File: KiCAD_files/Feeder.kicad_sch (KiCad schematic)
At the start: 61 parts, among them J505 Conn_01x03, Q501 60V N channel, Q502 TK13P25D,RQ, Q503 Q_Dual_NMOS_G1S2G2D2S1D1, Q504 Q_Dual_NMOS_G1S2G2D2S1D1, T501 PA2467NL, U501 NCP12700, U502 HMHA2801A, U503 TL431MFDT,215

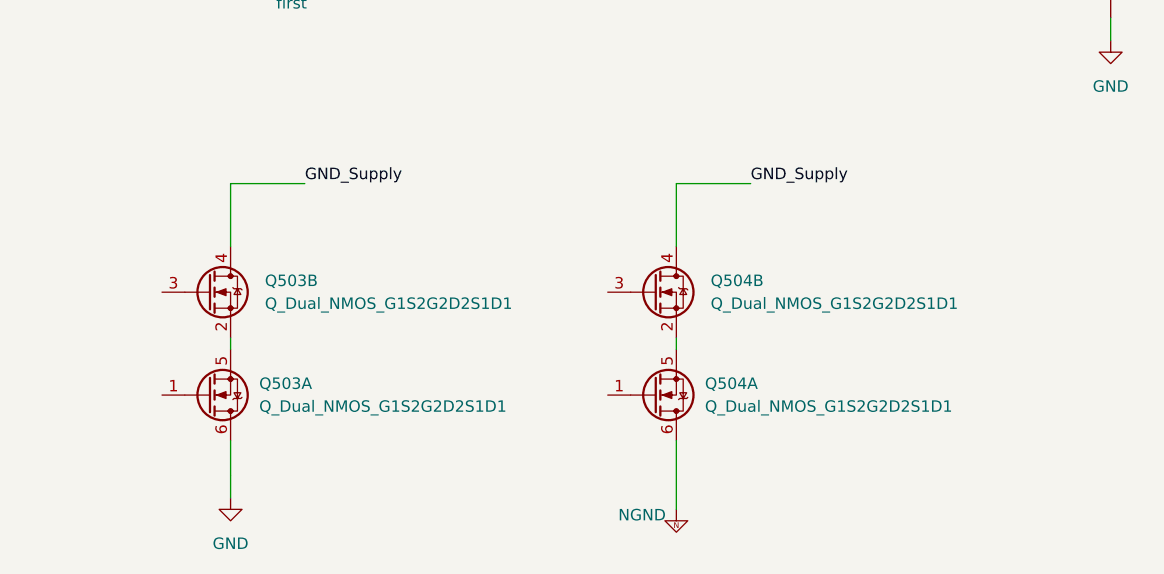
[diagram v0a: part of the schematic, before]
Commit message: Feature Freeze PCB ordered
Former-commit-id: 656e77d39b103ec58b17965582500bfb0a5b80a0
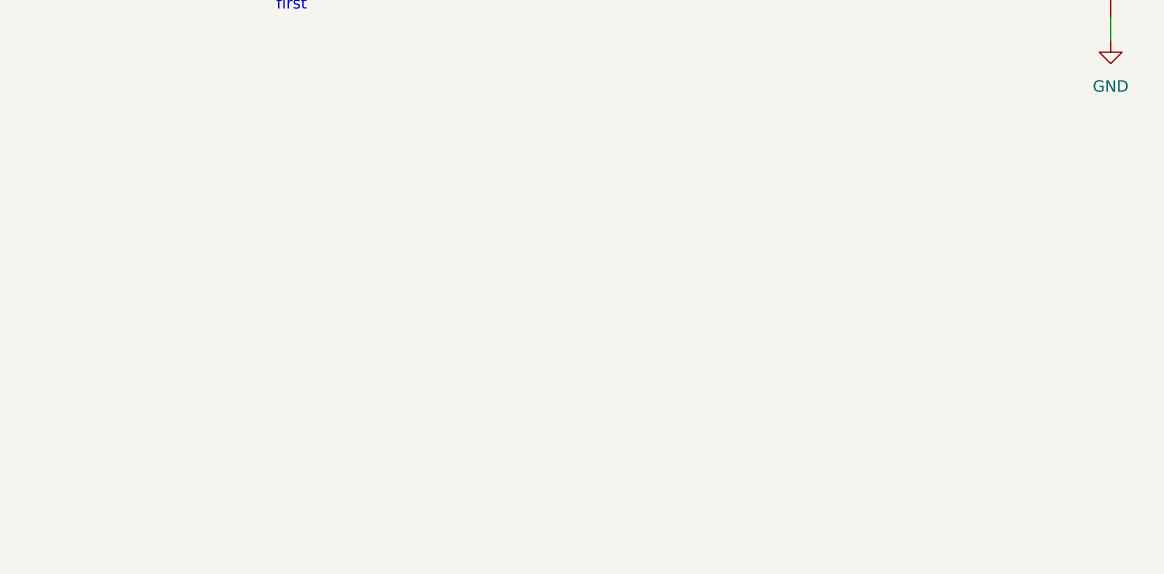
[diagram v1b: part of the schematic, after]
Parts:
- removed Q503, Q504: Q_Dual_NMOS_G1S2G2D2S1D1, symbol Device:Q_Dual_NMOS_G1S2G2D2S1D1
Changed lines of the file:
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@@
-    (stroke (width 0) (type default) (color 0 0 0 0))
-  )
-  (wire (pts (xy 71.755 223.52) (xy 71.755 224.79))
     (stroke (width 0) (type default) (color 0 0 0 0))
   )
@@
     (stroke (width 0) (type default) (color 0 0 0 0))
   )
-  (wire (pts (xy 121.285 234.95) (xy 121.285 238.76))
-    (stroke (width 0) (type default) (color 0 0 0 0))
-  )
   (wire (pts (xy 113.03 88.265) (xy 113.03 75.565))
     (stroke (width 0) (type default) (color 0 0 0 0))
@@
   )
   (wire (pts (xy 237.49 103.505) (xy 237.49 104.775))
-    (stroke (width 0.45) (type default) (color 0 0 0 0))
-  )
-  (wire (pts (xy 121.285 238.76) (xy 121.285 241.3))
     (stroke (width 0.45) (type default) (color 0 0 0 0))
   )
@@
     (stroke (width 0) (type default) (color 0 0 0 0))
   )
-  (wire (pts (xy 71.755 206.375) (xy 80.01 206.375))
-    (stroke (width 0) (type default) (color 0 0 0 0))
-  )
   (wire (pts (xy 196.85 104.775) (xy 205.105 104.775))
     (stroke (width 0) (type default) (color 0 0 0 0))
@@
     (stroke (width 0) (type default) (color 0 0 0 0))
   )
-  (wire (pts (xy 71.755 213.36) (xy 71.755 206.375))
-    (stroke (width 0) (type default) (color 0 0 0 0))
-  )
   (wire (pts (xy 180.975 94.615) (xy 180.975 90.805))
     (stroke (width 0) (type default) (color 0 0 0 0))
@@
   (wire (pts (xy 284.48 177.165) (xy 281.94 177.165))
     (stroke (width 0) (type default) (color 0 0 0 0))
-  )
-  (wire (pts (xy 71.755 238.76) (xy 71.755 241.3))
-    (stroke (width 0.45) (type default) (color 0 0 0 0))
   )
   (wire (pts (xy 162.56 125.73) (xy 162.56 139.7))
@@
     (stroke (width 0) (type default) (color 0 0 0 0))
   )
-  (wire (pts (xy 121.285 241.3) (xy 121.285 242.57))
-    (stroke (width 0) (type default) (color 0 0 0 0))
-  )
   (wire (pts (xy 180.975 104.775) (xy 196.85 104.775))
     (stroke (width 0) (type default) (color 0 0 0 0))
@@
     (stroke (width 0) (type default) (color 0 0 0 0))
   )
-  (wire (pts (xy 121.285 213.36) (xy 121.285 206.375))
-    (stroke (width 0) (type default) (color 0 0 0 0))
-  )
   (wire (pts (xy 222.885 24.13) (xy 222.885 26.035))
     (stroke (width 0) (type default) (color 0 0 0 0))
@@
   )
   (wire (pts (xy 90.17 139.7) (xy 90.17 146.05))
-    (stroke (width 0) (type default) (color 0 0 0 0))
-  )
-  (wire (pts (xy 121.285 206.375) (xy 129.54 206.375))
     (stroke (width 0) (type default) (color 0 0 0 0))
   )
@@
     (stroke (width 0.15) (type default) (color 0 0 0 0))
   )
-  (wire (pts (xy 71.755 234.95) (xy 71.755 238.76))
-    (stroke (width 0) (type default) (color 0 0 0 0))
-  )
   (wire (pts (xy 60.96 47.625) (xy 60.96 60.325))
     (stroke (width 0) (type default) (color 0 0 0 0))
@@
   )
   (wire (pts (xy 170.815 83.185) (xy 169.545 83.185))
-    (stroke (width 0) (type default) (color 0 0 0 0))
-  )
-  (wire (pts (xy 121.285 223.52) (xy 121.285 224.79))
     (stroke (width 0) (type default) (color 0 0 0 0))
   )
@@
     (effects (font (size 1.27 1.27)) (justify left bottom))
   )
-  (label "GND_Supply" (at 80.01 206.375 0)
-    (effects (font (size 1.27 1.27)) (justify left bottom))
-  )
   (label "+6VJP" (at 316.23 85.09 180)
     (effects (font (size 1.27 1.27)) (justify right bottom))
-  )
-  (label "GND_Supply" (at 129.54 206.375 0)
-    (effects (font (size 1.27 1.27)) (justify left bottom))
   )
   (label "VAUX" (at 187.96 124.46 0)
@@
     )
     (pin "1")
-  )
-  (symbol (lib_id "Device:Q_Dual_NMOS_G1S2G2D2S1D1") (at 118.745 229.87 0) (mirror x) (unit 1)
-    (in_bom yes) (on_board yes) (fields_autoplaced)
-    (property "Reference" "Q504" (id 0) (at 124.46 228.5999 0)
-      (effects (font (size 1.27 1.27)) (justify left))
-    )
-    (property "Value" "Q_Dual_NMOS_G1S2G2D2S1D1" (id 1) (at 124.46 231.1399 0)
-      (effects (font (size 1.27 1.27)) (justify left))
-    )
-    (property "Footprint" "" (id 2) (at 123.825 229.87 0)
-      (effects (font (size 1.27 1.27)) hide)
-    )
-    (property "Datasheet" "~" (id 3) (at 123.825 229.87 0)
-      (effects (font (size 1.27 1.27)) hide)
-    )
-    (pin "1")
-    (pin "5")
-    (pin "6")
   )
   (symbol (lib_id "Device:C") (at 229.87 38.735 90) (unit 1)
@@
     (pin "2")
   )
-  (symbol (lib_id "Device:Q_Dual_NMOS_G1S2G2D2S1D1") (at 69.215 229.87 0) (mirror x) (unit 1)
-    (in_bom yes) (on_board yes) (fields_autoplaced)
-    (property "Reference" "Q503" (id 0) (at 74.93 228.5999 0)
-      (effects (font (size 1.27 1.27)) (justify left))
-    )
-    (property "Value" "Q_Dual_NMOS_G1S2G2D2S1D1" (id 1) (at 74.93 231.1399 0)
-      (effects (font (size 1.27 1.27)) (justify left))
-    )
-    (property "Footprint" "" (id 2) (at 74.295 229.87 0)
-      (effects (font (size 1.27 1.27)) hide)
-    )
-    (property "Datasheet" "~" (id 3) (at 74.295 229.87 0)
-      (effects (font (size 1.27 1.27)) hide)
-    )
-    (pin "1")
-    (pin "5")
-    (pin "6")
-  )
   (symbol (lib_id "Device:Q_NMOS_GSD") (at 179.705 135.89 0) (mirror y) (unit 1)
     (in_bom yes) (on_board yes)
@@
     (pin "9")
   )
-  (symbol (lib_id "power:GND") (at 71.755 241.3 0) (unit 1)
-    (in_bom yes) (on_board yes)
-    (property "Reference" "#PWR0161" (id 0) (at 71.755 247.65 0)
-      (effects (font (size 1.27 1.27)) hide)
-    )
-    (property "Value" "GND" (id 1) (at 71.755 246.38 0))
-    (property "Footprint" "" (id 2) (at 71.755 241.3 0)
-      (effects (font (size 1.27 1.27)) hide)
-    )
-    (property "Datasheet" "" (id 3) (at 71.755 241.3 0)
-      (effects (font (size 1.27 1.27)) hide)
-    )
-    (pin "1")
-  )
   (symbol (lib_id "Device:L") (at 41.91 47.625 90) (unit 1)
     (in_bom yes) (on_board yes) (fields_autoplaced)
@@
     (pin "2")
   )
-  (symbol (lib_id "Symbols:NGND") (at 121.285 242.57 0) (unit 1)
-    (in_bom yes) (on_board yes)
-    (property "Reference" "#PWR0162" (id 0) (at 121.285 248.92 0)
-      (effects (font (size 1.27 1.27)) hide)
-    )
-    (property "Value" "NGND" (id 1) (at 117.475 243.205 0))
-    (property "Footprint" "" (id 2) (at 121.285 242.57 0)
-      (effects (font (size 1.27 1.27)) hide)
-    )
-    (property "Datasheet" "" (id 3) (at 121.285 242.57 0)
-      (effects (font (size 1.27 1.27)) hide)
-    )
-    (pin "1")
-  )
   (symbol (lib_id "Device:C") (at 35.56 64.135 0) (unit 1)
     (in_bom yes) (on_board yes)
@@
     (pin "2")
   )
-  (symbol (lib_id "Device:Q_Dual_NMOS_G1S2G2D2S1D1") (at 69.215 218.44 0) (unit 2)
-    (in_bom yes) (on_board yes) (fields_autoplaced)
-    (property "Reference" "Q503" (id 0) (at 75.565 217.1699 0)
-      (effects (font (size 1.27 1.27)) (justify left))
-    )
-    (property "Value" "Q_Dual_NMOS_G1S2G2D2S1D1" (id 1) (at 75.565 219.7099 0)
-      (effects (font (size 1.27 1.27)) (justify left))
-    )
-    (property "Footprint" "" (id 2) (at 74.295 218.44 0)
-      (effects (font (size 1.27 1.27)) hide)
-    )
-    (property "Datasheet" "~" (id 3) (at 74.295 218.44 0)
-      (effects (font (size 1.27 1.27)) hide)
-    )
-    (pin "2")
-    (pin "3")
-    (pin "4")
-  )
   (symbol (lib_id "Symbols:V1.1.2") (at 105.41 88.9 0) (unit 1)
     (in_bom yes) (on_board yes)
@@
     (pin "2")
   )
-  (symbol (lib_id "Device:Q_Dual_NMOS_G1S2G2D2S1D1") (at 118.745 218.44 0) (unit 2)
-    (in_bom yes) (on_board yes) (fields_autoplaced)
-    (property "Reference" "Q504" (id 0) (at 125.095 217.1699 0)
-      (effects (font (size 1.27 1.27)) (justify left))
-    )
-    (property "Value" "Q_Dual_NMOS_G1S2G2D2S1D1" (id 1) (at 125.095 219.7099 0)
-      (effects (font (size 1.27 1.27)) (justify left))
-    )
-    (property "Footprint" "" (id 2) (at 123.825 218.44 0)
-      (effects (font (size 1.27 1.27)) hide)
-    )
-    (property "Datasheet" "~" (id 3) (at 123.825 218.44 0)
-      (effects (font (size 1.27 1.27)) hide)
-    )
-    (pin "2")
-    (pin "3")
-    (pin "4")
-  )
   (symbol (lib_id "Symbols:V1.1.2") (at 292.1 184.15 0) (unit 1)
